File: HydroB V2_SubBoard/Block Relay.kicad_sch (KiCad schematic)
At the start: 40 parts, among them J10 Screw_Terminal_01x02, J16 Screw_Terminal_01x02, J3 Screw_Terminal_01x02, J8 Screw_Terminal_01x02, J9 Screw_Terminal_01x02, Q1 S8050, Q2 S8050, Q3 S8050, Q4 S8050, Q5 S8050

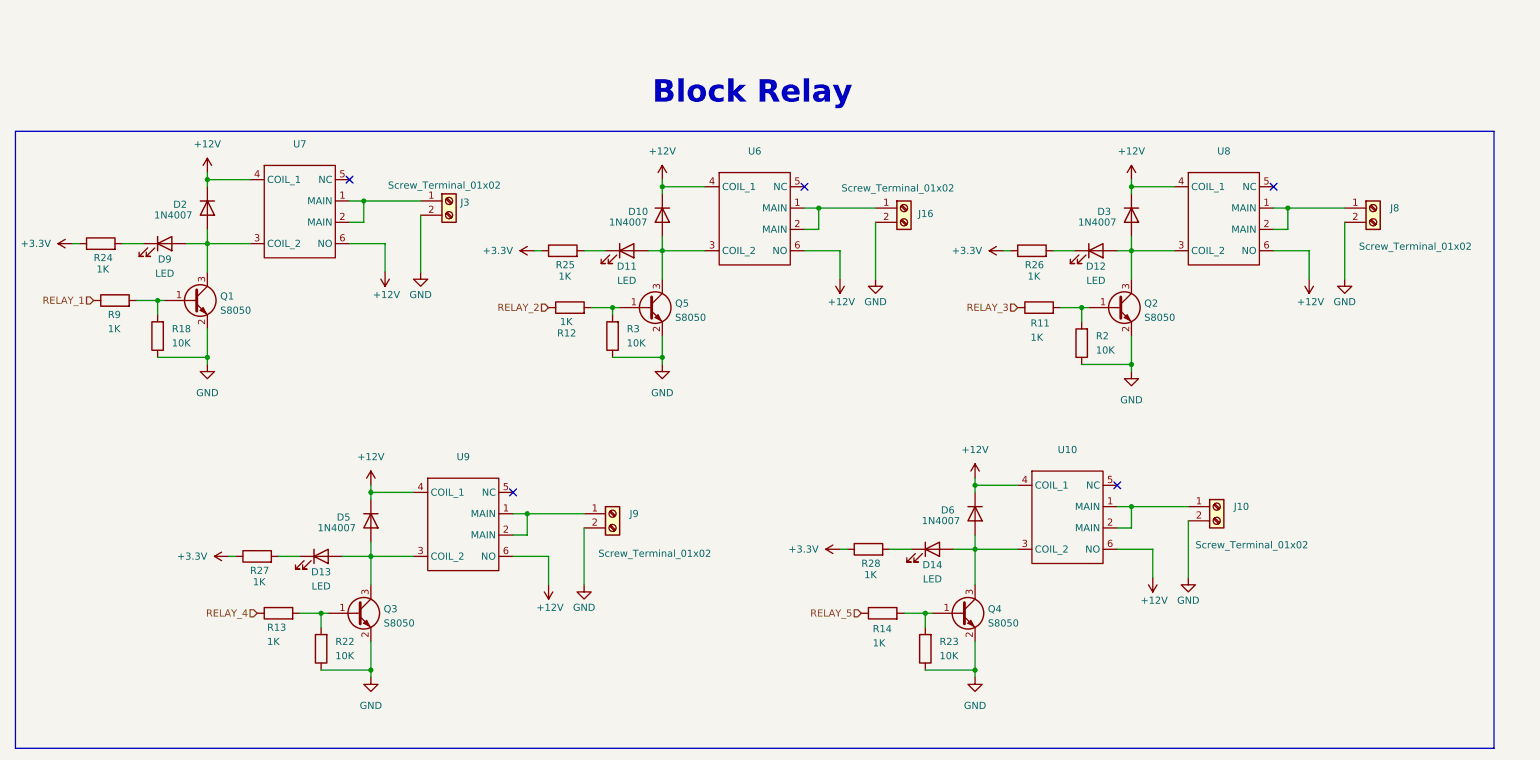
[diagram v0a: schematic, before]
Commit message: PCB update
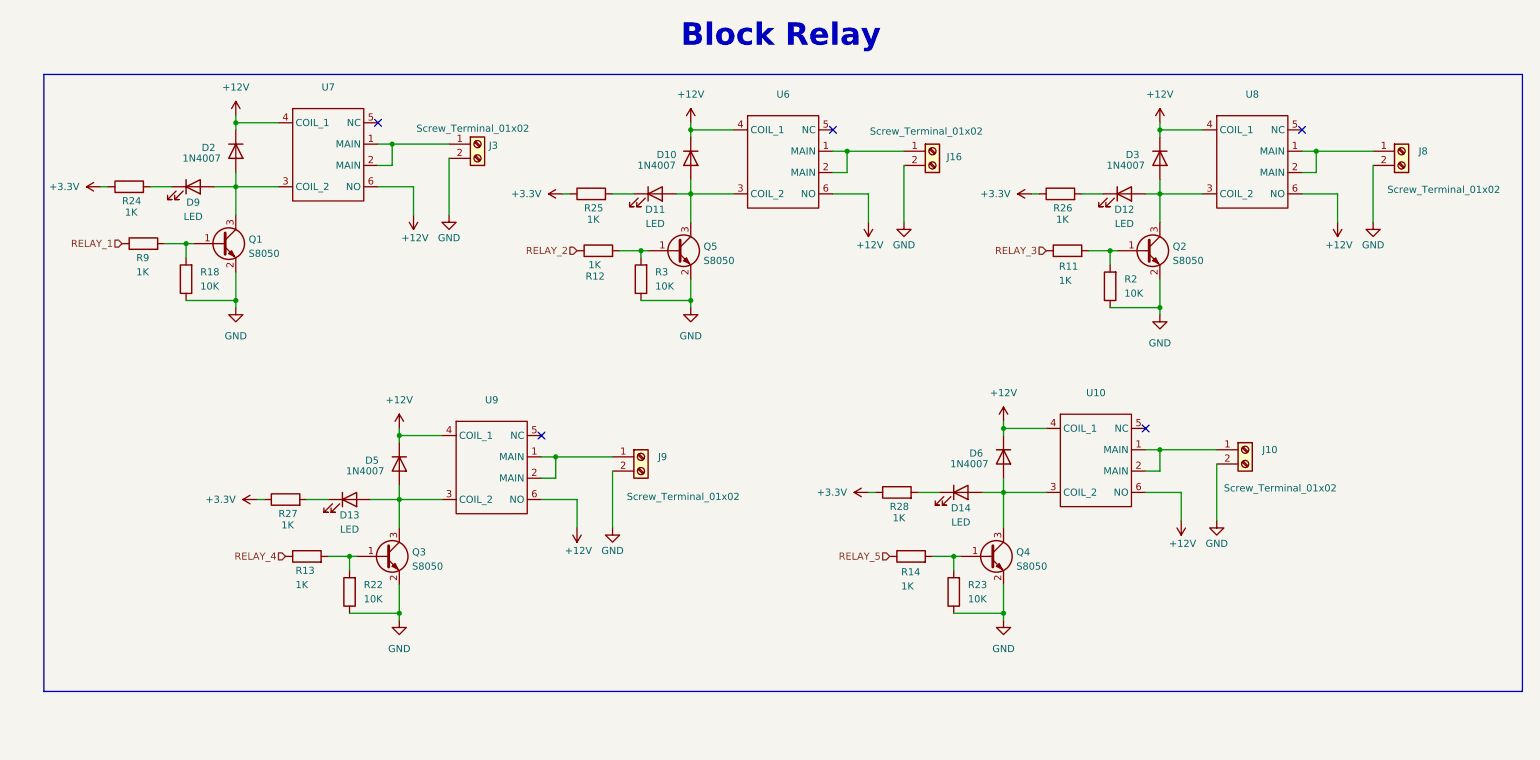
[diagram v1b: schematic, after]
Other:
- moved on the sheet: D10, D11, D12, D13, D14, D2, D3, D5, D6, D9, J10, J16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
